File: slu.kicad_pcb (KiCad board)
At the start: 2 copper layers, 99.6 x 100.9 mm, 168 parts, among them J1 lcd_out, sw1 sw_2pos

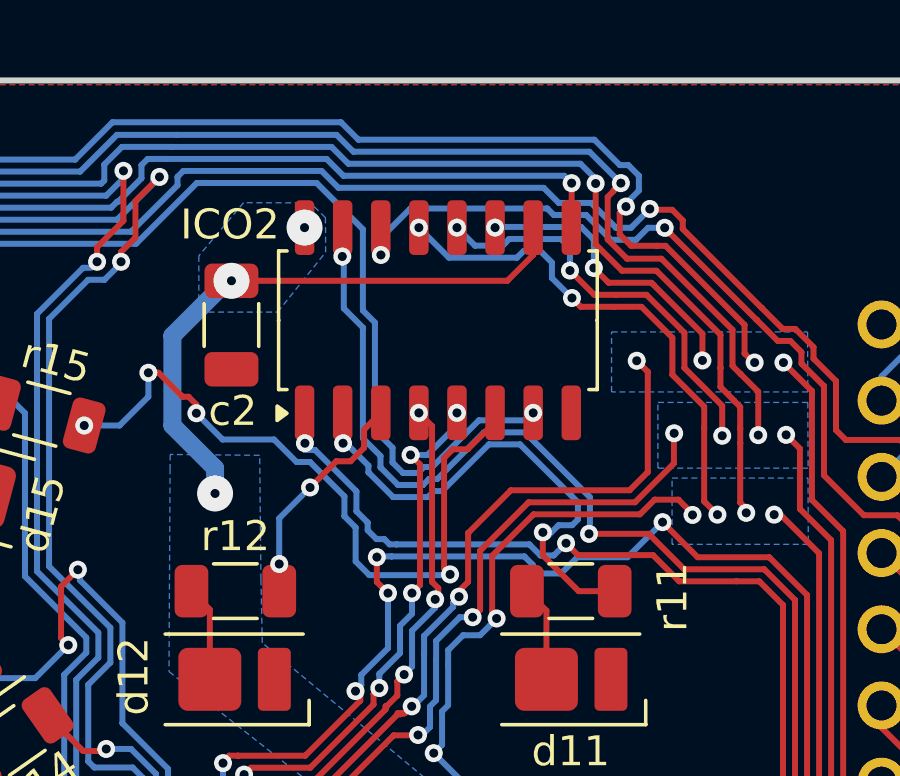
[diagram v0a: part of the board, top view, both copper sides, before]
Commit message: started ico2 cleanup
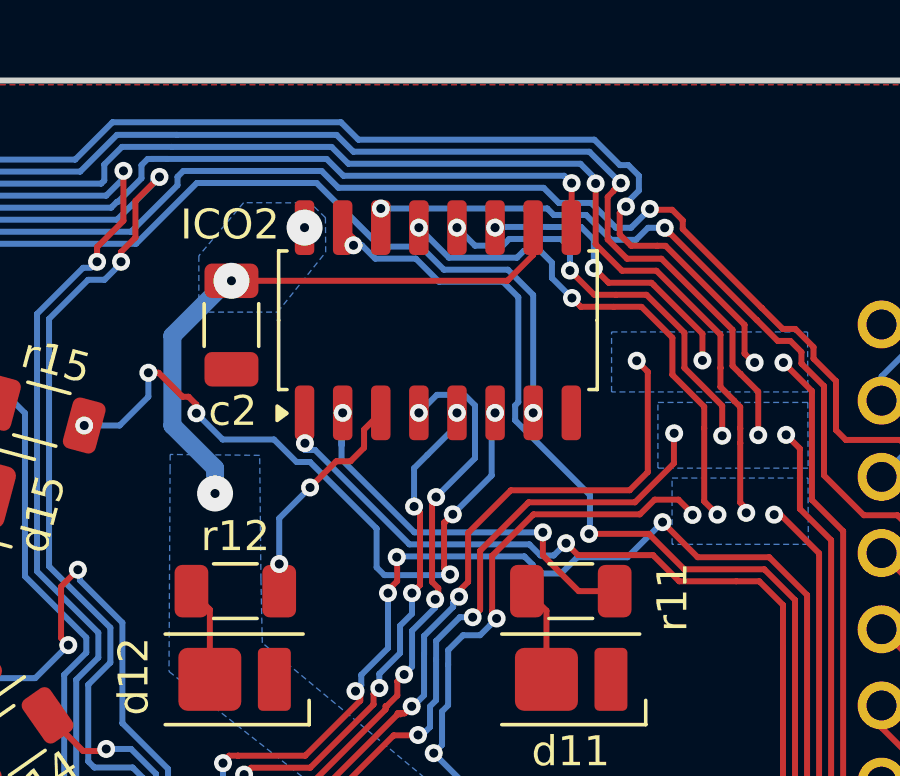
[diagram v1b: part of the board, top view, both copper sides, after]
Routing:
- net /ICD11: track 17.0 -> 13.7 mm
- net /ICD13: track 31.8 -> 34.7 mm, vias 5 -> 6
- net /ICD9: track 48.6 -> 46.0 mm
- net /SER1-2: track 96.9 -> 94.8 mm
- net /ICD16: track 30.4 -> 28.7 mm
- net /ICD63: track 106.8 -> 106.1 mm
- net /ICD10: track 33.5 -> 33.0 mm
- net /ICD15: track 25.2 -> 25.0 mm, vias 4 -> 6
